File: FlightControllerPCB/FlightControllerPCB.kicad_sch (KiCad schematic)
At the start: 0 parts

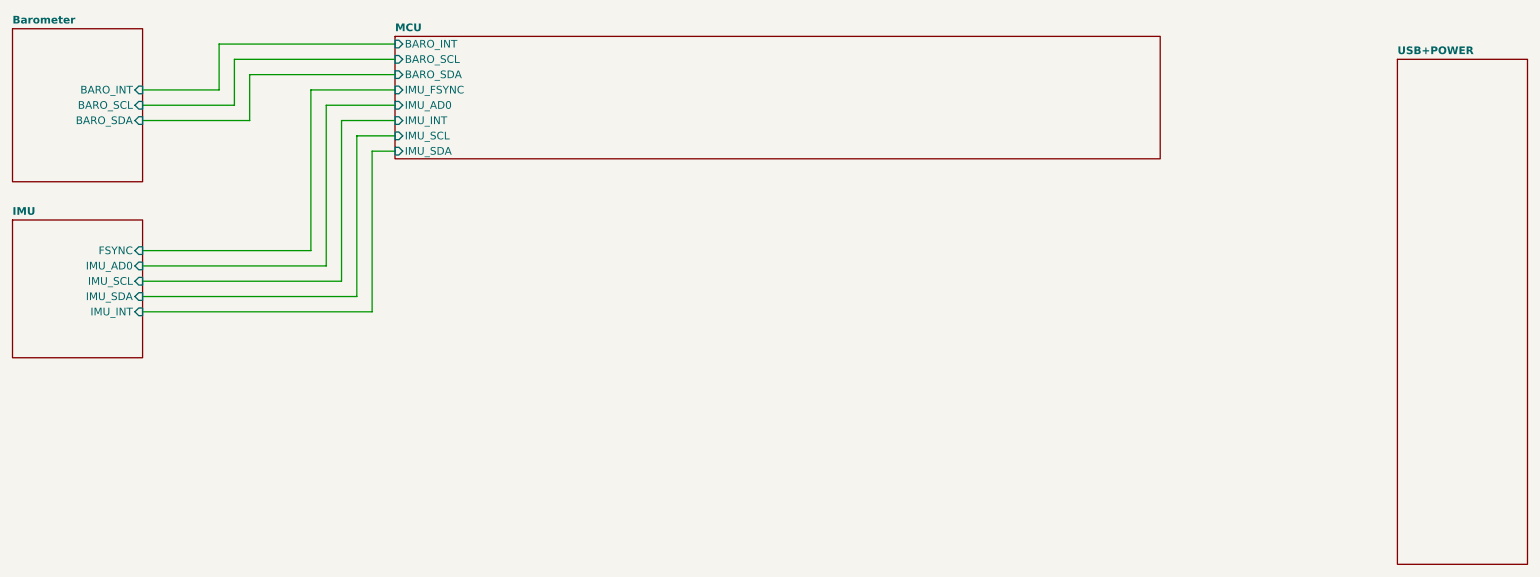
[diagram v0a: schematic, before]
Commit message: early MCU setup
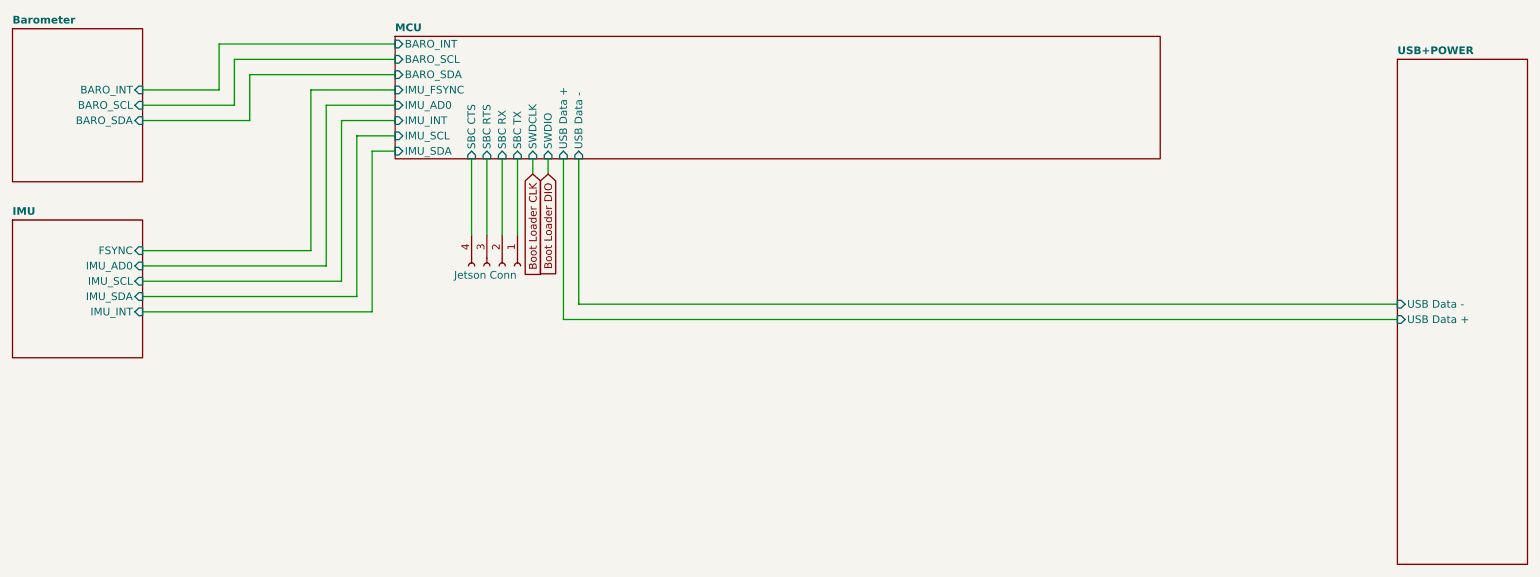
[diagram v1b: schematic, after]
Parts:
- added J2: Jetson Conn, symbol Connector:Conn_01x04_Socket
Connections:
- new net MCU/SBC CTS: J2.4 (Pin_4)
- new net MCU/SBC RTS: J2.3 (Pin_3)
- new net MCU/SBC RX: J2.2 (Pin_2)
- new net MCU/SBC TX: J2.1 (Pin_1)
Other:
- sheet MCU ports: added SBC CTS, SBC RTS, SBC RX, SBC TX, SWDCLK, SWDIO, USB Data +, USB Data -; removed none
- sheet USB+POWER ports: added USB Data +, USB Data -; removed none
